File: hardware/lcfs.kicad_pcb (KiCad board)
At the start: 2 copper layers, 58.2 x 15.2 mm, 8 parts, among them J3 Pin_1x2_Battery, J4 Pin_1x3_Transmitter

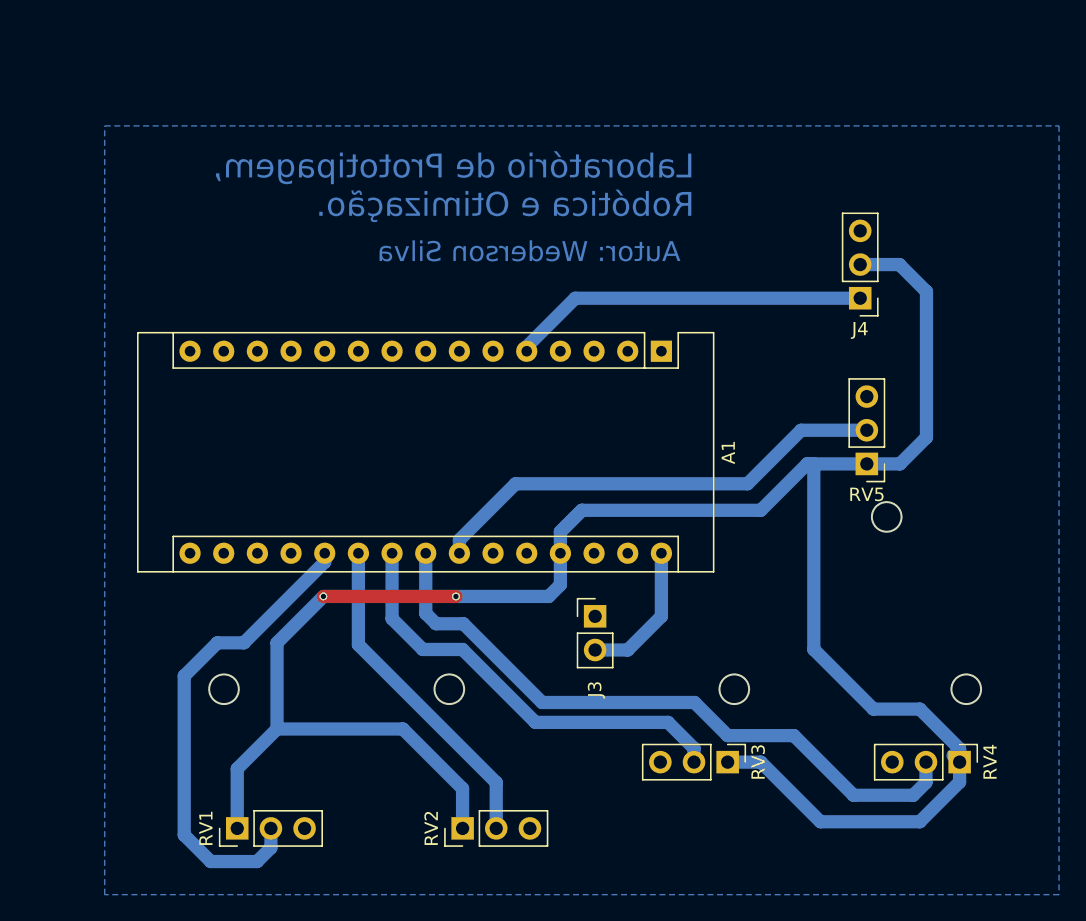
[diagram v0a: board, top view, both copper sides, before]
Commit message: v0.1.15 Renomeia valores
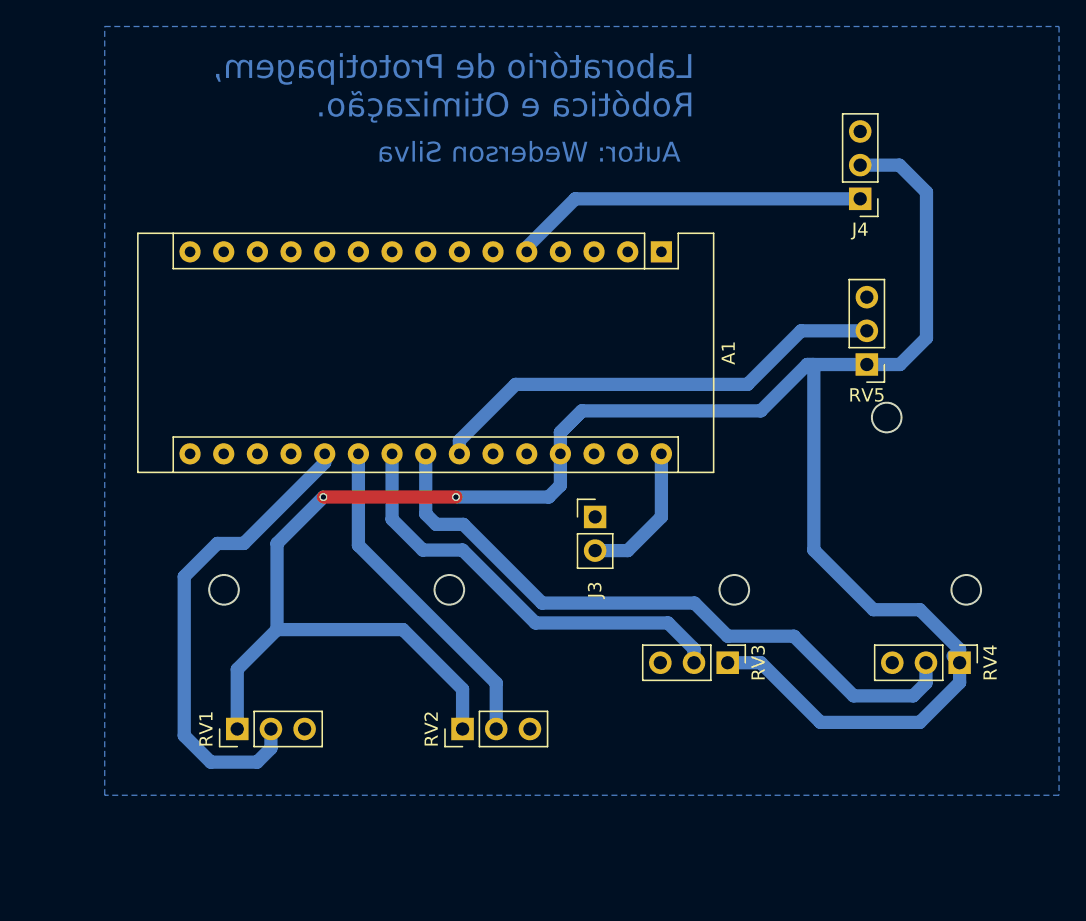
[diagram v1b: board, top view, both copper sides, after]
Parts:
- moved A1 7.50 mm to (219.0, 125.0)
- moved J3 7.50 mm to (214.0, 145.0)
- moved J4 7.50 mm to (234.0, 121.0)
- moved RV1 7.50 mm to (187.0, 161.0)
- moved RV2 7.50 mm to (204.0, 161.0)
- moved RV3 7.50 mm to (224.0, 156.0)
- moved RV4 7.50 mm to (241.5, 156.0)
- moved RV5 7.50 mm to (234.5, 133.5)
